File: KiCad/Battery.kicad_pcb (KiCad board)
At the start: 2 copper layers, 19 x 29 mm, 26 parts, among them J1 Connector, J2 USB-C, J3 DC, Q1 RN1701, U1 ESP32-WROOM-32, U2 FT231XQ, U3 NX6020CAKS

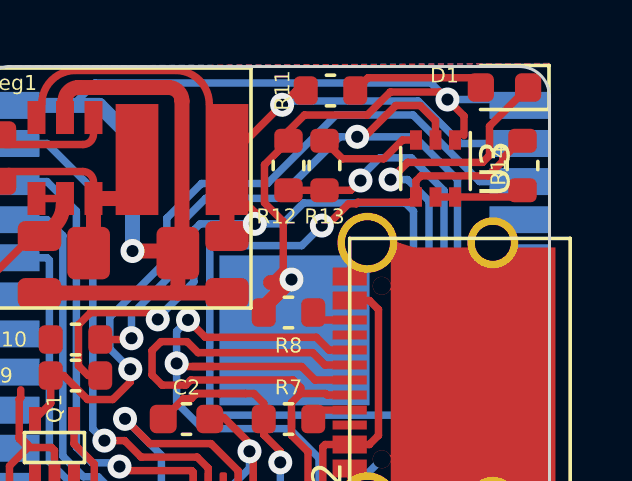
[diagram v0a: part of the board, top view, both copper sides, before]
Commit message: Tidy drawing
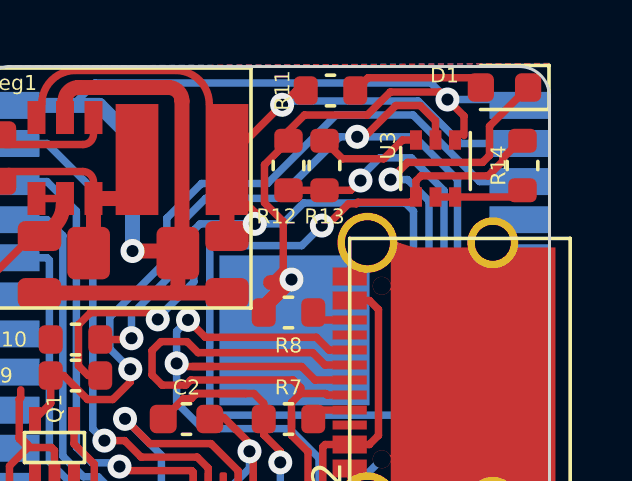
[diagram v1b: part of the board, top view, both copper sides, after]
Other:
- board text added: "22"
- board text added: "23"
- board text added: "25"
- board text added: "32"
- board text added: "33"
